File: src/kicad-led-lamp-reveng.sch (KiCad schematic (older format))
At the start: 18 parts, among them J1 AC2, J2 AC1, J3 L+, J4 L-, SW1 SW_Push_SPDT

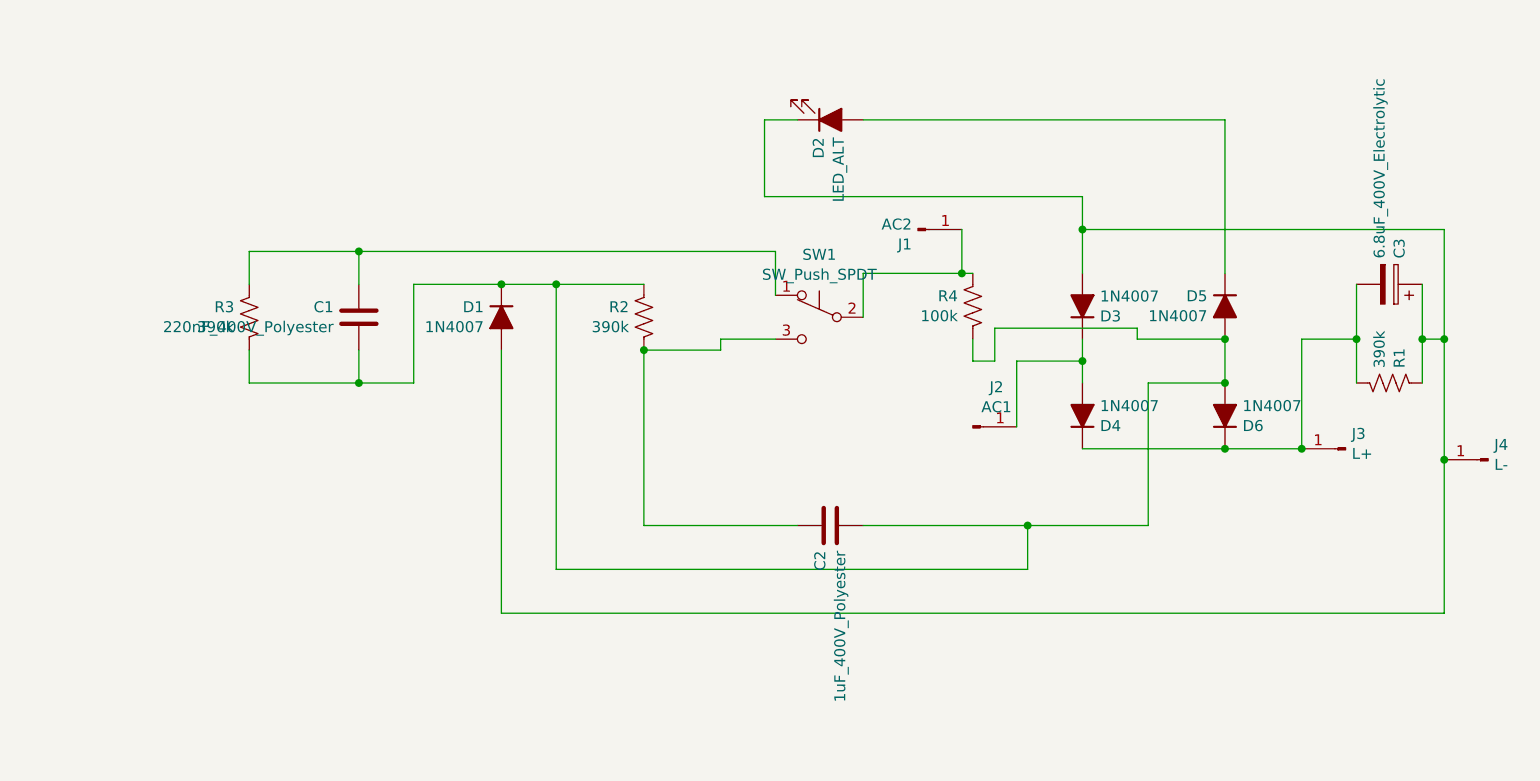
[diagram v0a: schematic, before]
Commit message: Finished pcb layout
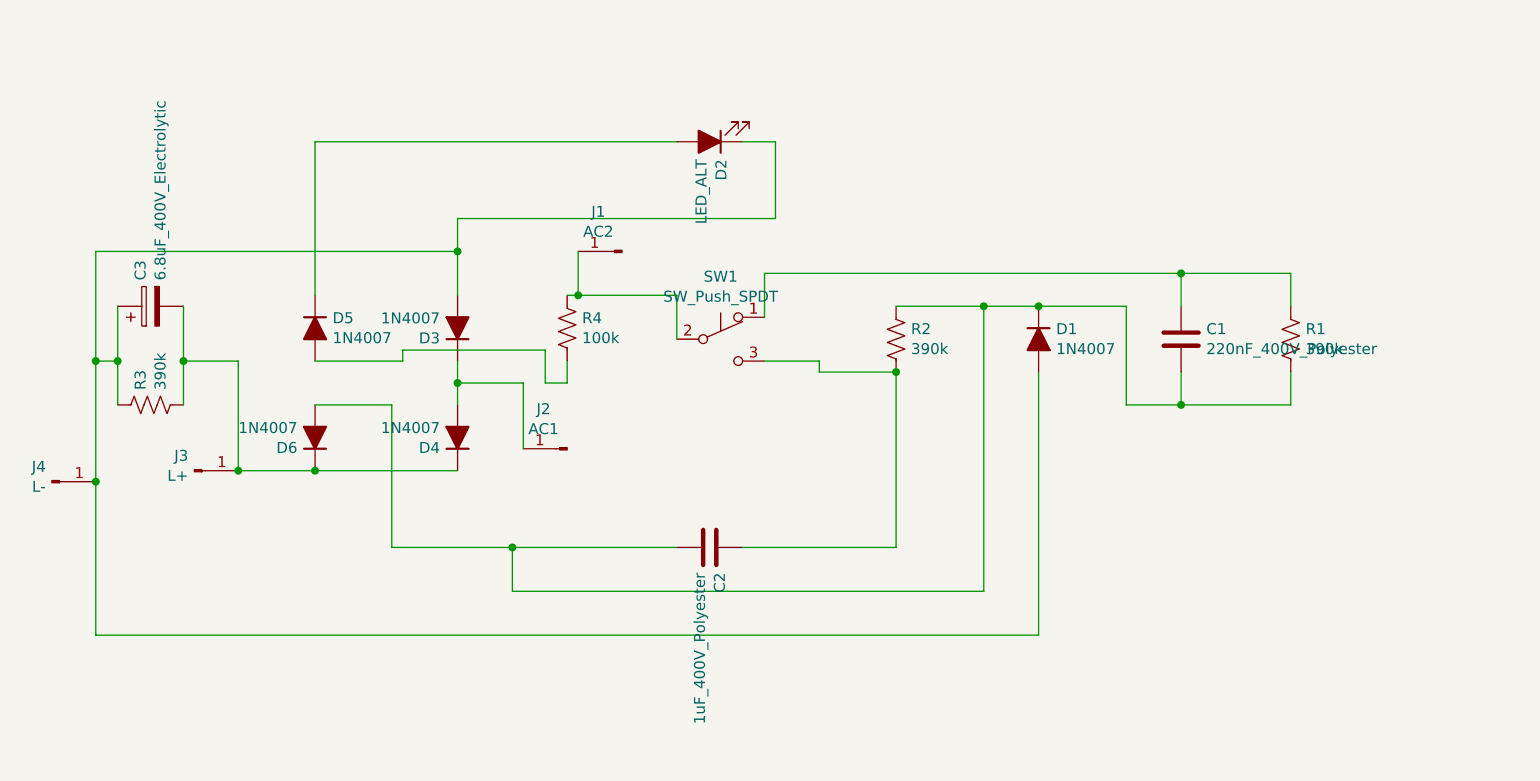
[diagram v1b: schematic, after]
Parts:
- C1: footprint (none) -> igorkelvin:C_Polyester_11.20mm_4.9mm
- C2: footprint (none) -> igorkelvin:C_Polyester_21.80mm_7.10mm
- D1, D3, D4, D5, D6: footprint Resistor_THT:R_Axial_DIN0207_L6.3mm_D2.5mm_P7.62mm_Horizontal -> igorkelvin:DIODE_Axial_DIN0207_L6.3mm_D2.5mm_P7.62mm_Horizontal
- J1, J2, J3, J4: footprint (none) -> Connector_PinHeader_2.54mm:PinHeader_1x01_P2.54mm_Vertical
- SW1: footprint (none) -> igorkelvin:Switch_4-Way
- renumbered R3 to R1, R1 to R3
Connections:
- net at C1.2, C2.2, D1.1 (K)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: no longer D5.2 (A), R4.2
- new net: D5.2 (A), R4.2
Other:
- moved on the sheet: C1, C2, C3, D1, D2, D3, D4, D5, D6, J1, J2, J3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

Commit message: Schematics rearrangement, changed C3 polarity and Rev1 for pcb & sch
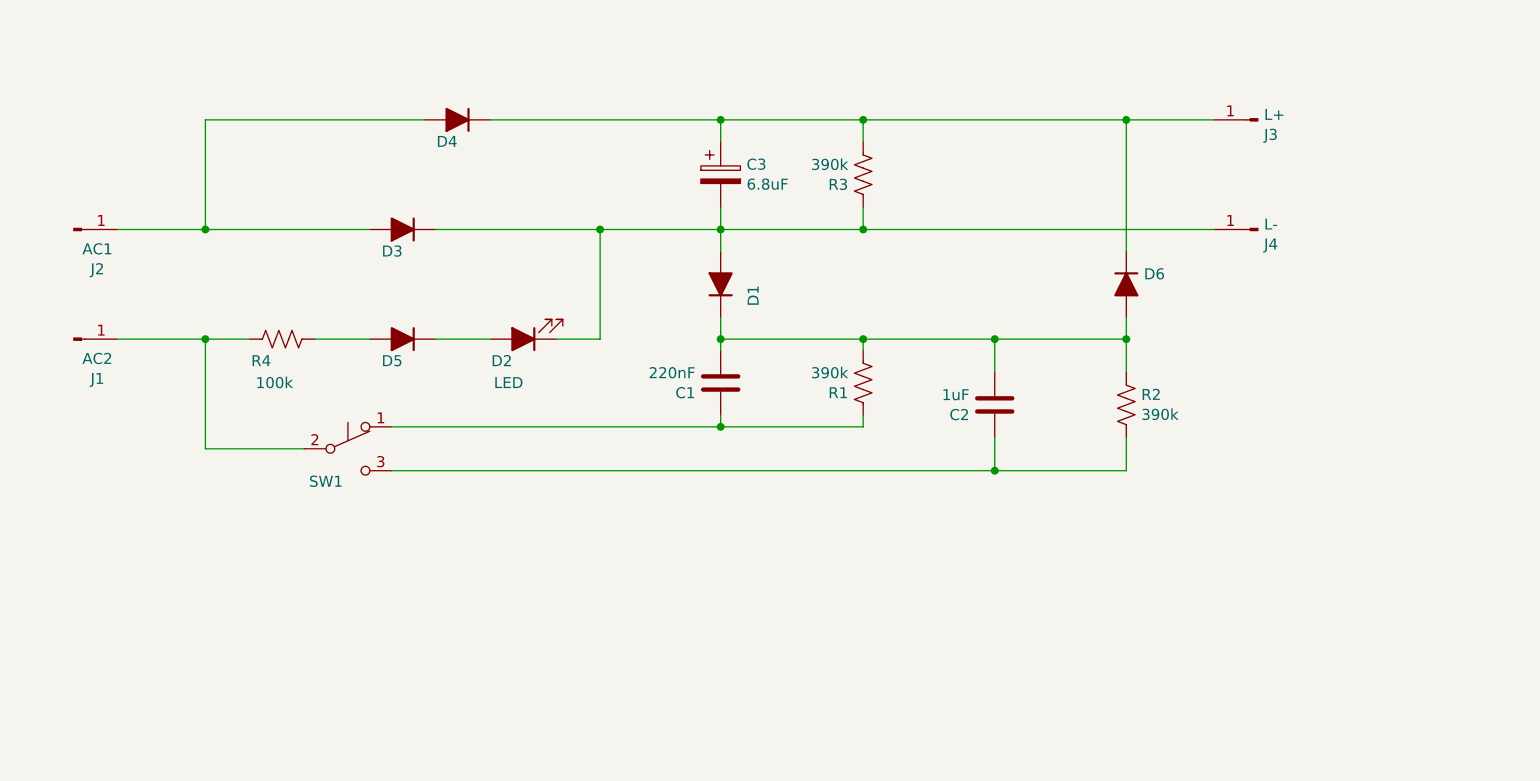
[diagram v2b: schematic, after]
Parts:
- C1: value 220nF_400V_Polyester -> 220nF
- C2: value 1uF_400V_Polyester -> 1uF
- C3: value 6.8uF_400V_Electrolytic -> 6.8uF
- D2: value LED_ALT -> LED
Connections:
- net at D1.2 (A), D2.1 (K), J4.1 (Pin_1)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: now also C3.2, D3.1 (K); no longer C3.1, D3.2 (A)
- net at D4.1 (K), D6.1 (K), J3.1 (Pin_1)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: now also C3.1; no longer C3.2
- net at D4.2 (A), J2.1 (Pin_1): now also D3.2 (A); no longer D3.1 (K)
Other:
- moved on the sheet: C1, C2, C3, D1, D2, D3, D4, D5, D6, J1, J2, J3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
